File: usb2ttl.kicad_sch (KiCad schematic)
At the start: 10 parts, among them Q1 BSS138, Q2 BSS138, U2 CH340C

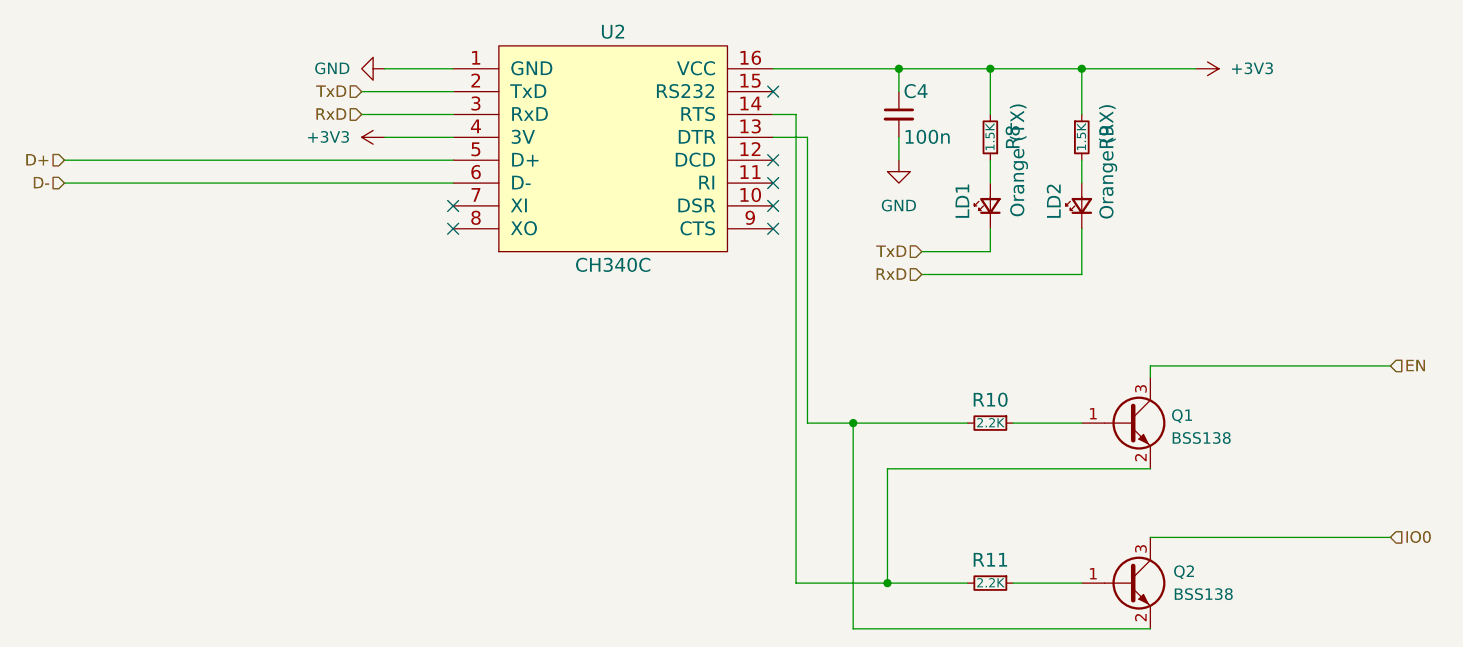
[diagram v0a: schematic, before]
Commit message: HW 1.06 WIP
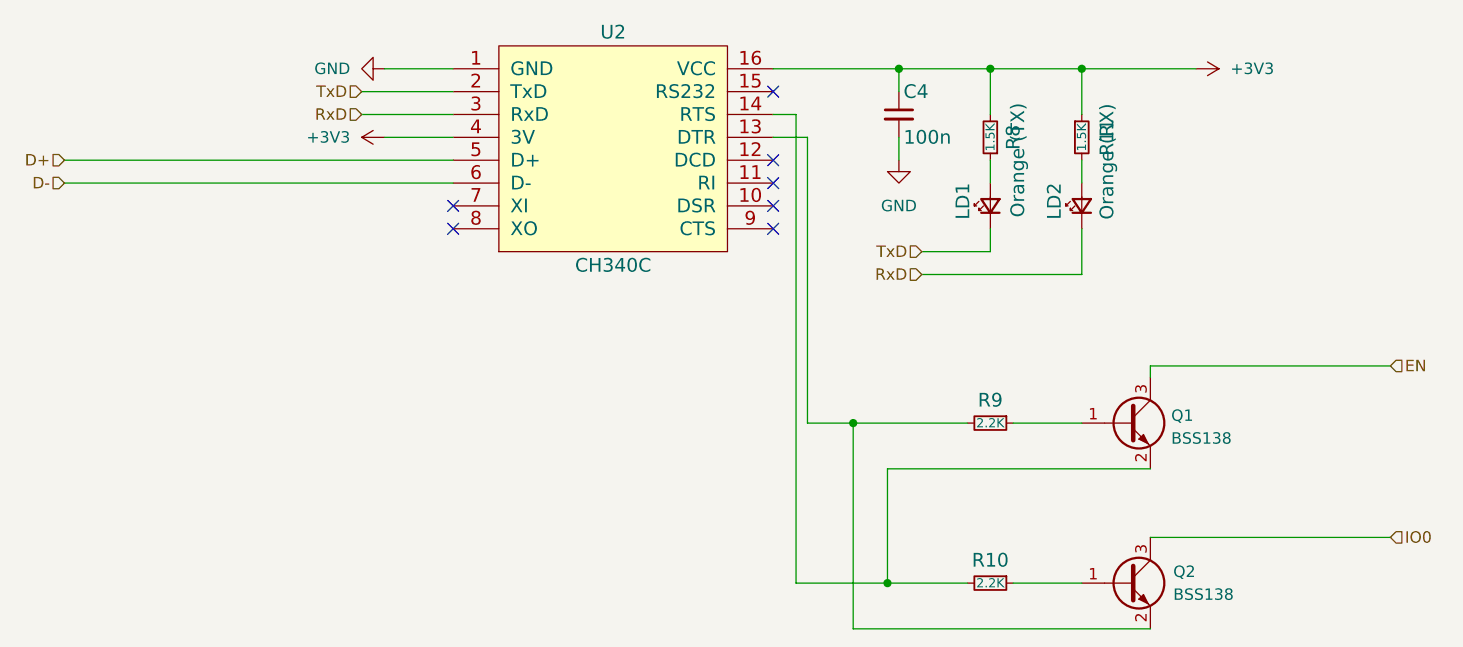
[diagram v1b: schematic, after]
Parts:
- renumbered R11 to R10, R9 to R11, R10 to R9
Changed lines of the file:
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@@
 		(dnp no)
 		(fields_autoplaced yes)
-		(property "Reference" "#PWR019"
+		(property "Reference" "#PWR018"
 			(at 121.92 74.93 0)
 			(effects
@@
 			(project "echo"
 				(path "/8c0b3d8b-46d3-4173-ab1e-a61765f77d61/f883457e-0c9e-4a1d-9f19-b038d36f033f"
-					(reference "#PWR019")
+					(reference "#PWR018")
 					(unit 1)
 				)
@@
 		(dnp no)
 		(fields_autoplaced yes)
-		(property "Reference" "#PWR018"
+		(property "Reference" "#PWR020"
 			(at 204.47 67.31 0)
 			(effects
@@
 			(project ""
 				(path "/8c0b3d8b-46d3-4173-ab1e-a61765f77d61/f883457e-0c9e-4a1d-9f19-b038d36f033f"
-					(reference "#PWR018")
+					(reference "#PWR020")
 					(unit 1)
 				)
@@
 		(on_board yes)
 		(dnp no)
-		(property "Reference" "R10"
+		(property "Reference" "R9"
 			(at 185.42 104.14 90)
 			(effects
@@
 			(project "echo"
 				(path "/8c0b3d8b-46d3-4173-ab1e-a61765f77d61/f883457e-0c9e-4a1d-9f19-b038d36f033f"
-					(reference "R10")
+					(reference "R9")
 					(unit 1)
 				)
@@
 		(on_board yes)
 		(dnp no)
-		(property "Reference" "R9"
+		(property "Reference" "R11"
 			(at 198.374 74.93 90)
 			(effects
@@
 			(project "echo"
 				(path "/8c0b3d8b-46d3-4173-ab1e-a61765f77d61/f883457e-0c9e-4a1d-9f19-b038d36f033f"
-					(reference "R9")
+					(reference "R11")
 					(unit 1)
 				)
@@
 		(on_board yes)
 		(dnp no)
-		(property "Reference" "#PWR020"
+		(property "Reference" "#PWR019"
 			(at 175.26 83.82 0)
 			(effects
@@
 			(project "echo"
 				(path "/8c0b3d8b-46d3-4173-ab1e-a61765f77d61/f883457e-0c9e-4a1d-9f19-b038d36f033f"
-					(reference "#PWR020")
+					(reference "#PWR019")
 					(unit 1)
 				)
@@
 		(on_board yes)
 		(dnp no)
-		(property "Reference" "R11"
+		(property "Reference" "R10"
 			(at 185.42 121.92 90)
 			(effects
@@
 			(project "echo"
 				(path "/8c0b3d8b-46d3-4173-ab1e-a61765f77d61/f883457e-0c9e-4a1d-9f19-b038d36f033f"
-					(reference "R11")
-					(unit 1)
-				)
+					(reference "R10")
+					(unit 1)
+				)
